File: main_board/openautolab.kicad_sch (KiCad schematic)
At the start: 32 parts, among them J1 PIN11, J10 HX711, J11 LCD, J12 OUT+, J13 OUT-, J14 IN+, J15 IN-, J16 PWR_IN, J17 FILTER_PUMP, J18 FILTER_SENSOR, J2 PIN9, J3 PIN10, J4 PIN12, J6 PIN7, J7 PIN8, J8 PUMP, J9 SERVO, K1 FINDER-36.11, K2 FINDER-36.11, SW0 PIN_A0, SW1 PIN_A1, SW2 PIN_A2, SW3 SW_SPDT, U1 TD62064APG, U2 TD62064APG

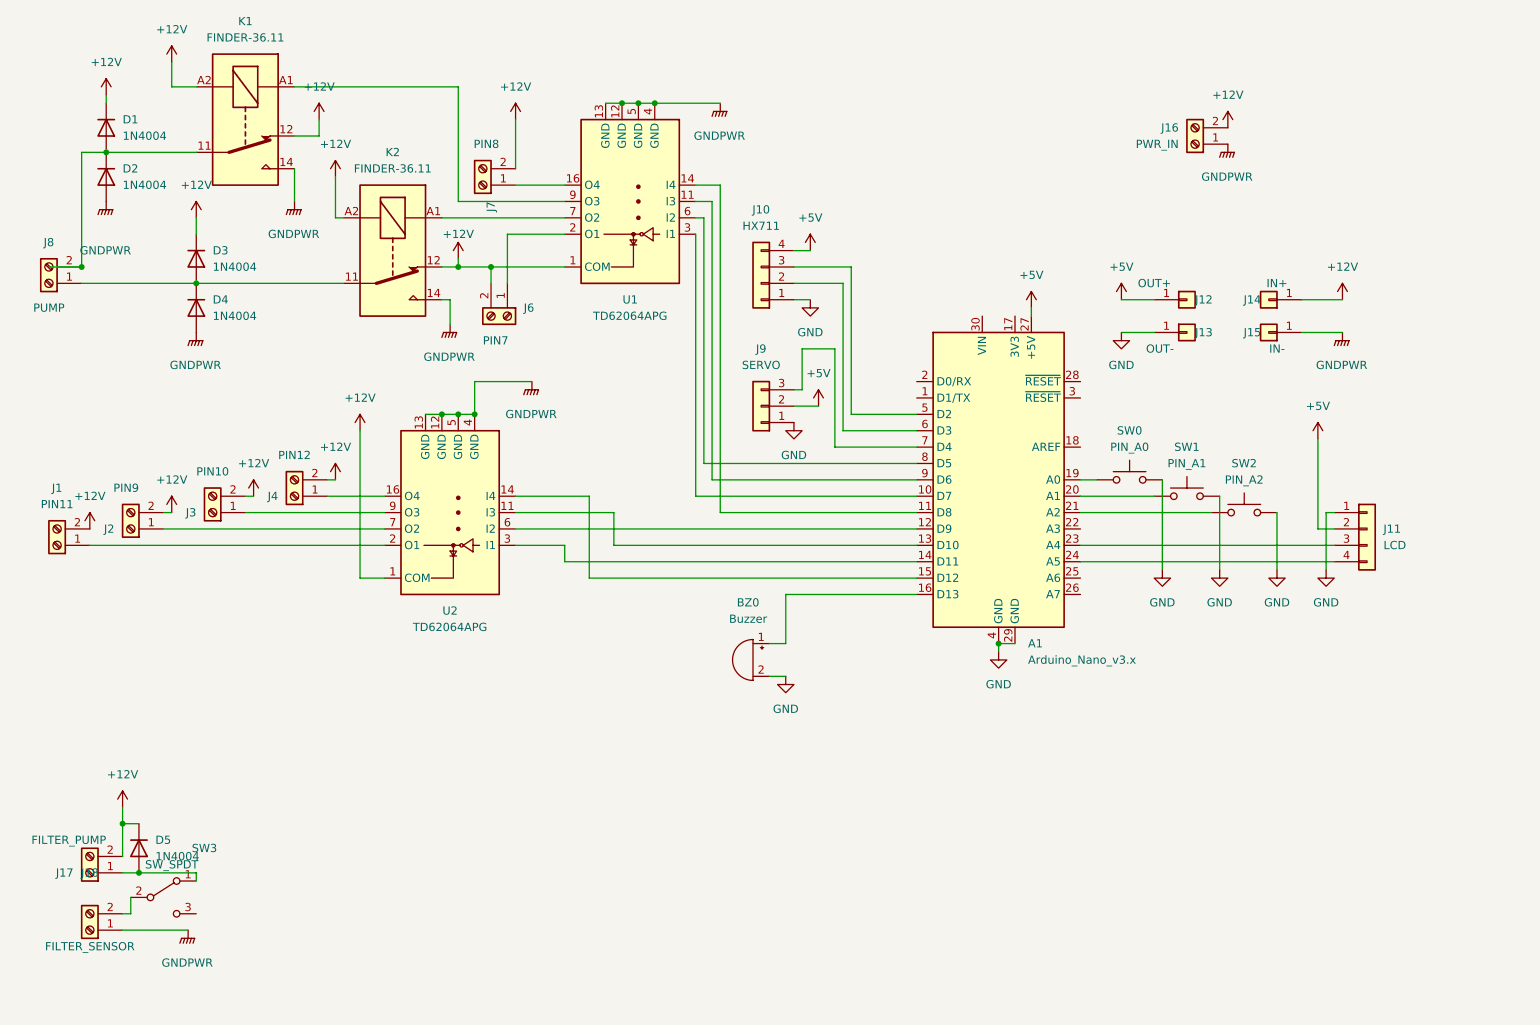
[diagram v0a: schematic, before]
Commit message: update PCB
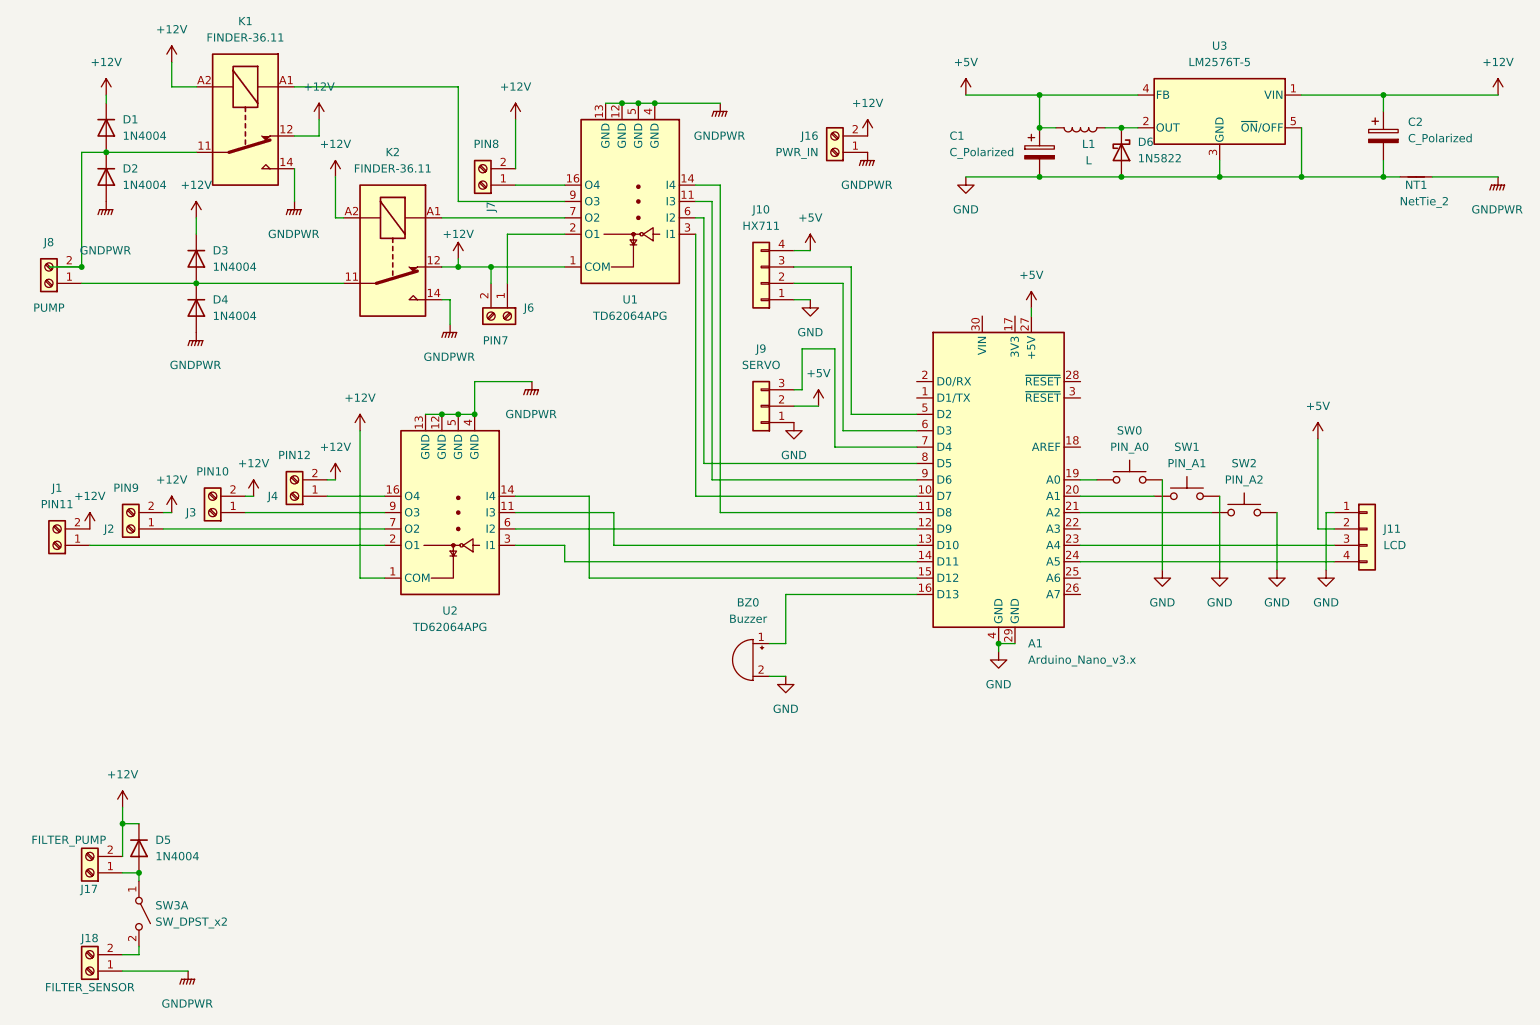
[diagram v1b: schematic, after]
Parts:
- removed J12: OUT+, Connector_PinHeader_2.54mm:PinHeader_1x01_P2.54mm_Vertical, symbol Connector_Generic:Conn_01x01
- removed J13: OUT-, Connector_PinHeader_2.54mm:PinHeader_1x01_P2.54mm_Vertical, symbol Connector_Generic:Conn_01x01
- removed J14: IN+, Connector_PinHeader_2.54mm:PinHeader_1x01_P2.54mm_Vertical, symbol Connector_Generic:Conn_01x01
- removed J15: IN-, Connector_PinHeader_2.54mm:PinHeader_1x01_P2.54mm_Vertical, symbol Connector_Generic:Conn_01x01
- removed SW3: SW_SPDT, Button_Switch_THT:SW_Slide_1P2T_CK_OS102011MS2Q, symbol Switch:SW_SPDT
- added C1: C_Polarized, Capacitor_THT:CP_Radial_D10.0mm_P5.00mm, symbol Device:C_Polarized
- added C2: C_Polarized, Capacitor_THT:CP_Radial_D8.0mm_P5.00mm, symbol Device:C_Polarized
- added D6: 1N5822, Diode_THT:D_DO-201AD_P15.24mm_Horizontal, symbol Diode:1N5822
- added L1: L, Inductor_THT:L_Toroid_Vertical_L26.7mm_W14.0mm_P10.16mm_Pulse_D, symbol Device:L
- added NT1: NetTie_2, NetTie:NetTie-2_SMD_Pad2.0mm, symbol Device:NetTie_2
- added SW3: SW_DPST_x2, Connector_PinHeader_2.54mm:PinHeader_1x02_P2.54mm_Vertical, symbol Switch:SW_DPST_x2
- added U3: LM2576T-5, Package_TO_SOT_THT:TO-220-5_Vertical, symbol Regulator_Switching:LM2576T-5
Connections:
- net +12V: now also C2.1, U3.1 (VIN)
- net +5V: now also C1.1, L1.2, U3.4 (FB)
- net GND: now also C1.2, C2.2, D6.2 (A), NT1.1, U3.3 (GND), U3.5 (~{ON}/OFF)
- net GNDPWR: now also NT1.2
- net at J18.2 (Pin_2): now also SW3.2 (B)
- net at D5.2 (A), J17.1 (Pin_1): now also SW3.1 (A)
- new net: D6.1 (K), L1.1, U3.2 (OUT)
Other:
- moved on the sheet: J16, J18
